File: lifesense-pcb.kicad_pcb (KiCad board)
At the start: 2 copper layers, 56 parts, among them CON1 USB-MINI-B, IC1 CC3000, J1 CONN_10X2, J4 CONN_10X2, P1 CONN_6, P2 CONN_01X01, P21 CONN_01X01, Q1 DTC114E, Q2 DTC114E, Q3 DTC114E, U1 TM4C123GH6PM, U2 TPS73633DRB, Y1 CRYSTAL, Y2 CRYSTAL

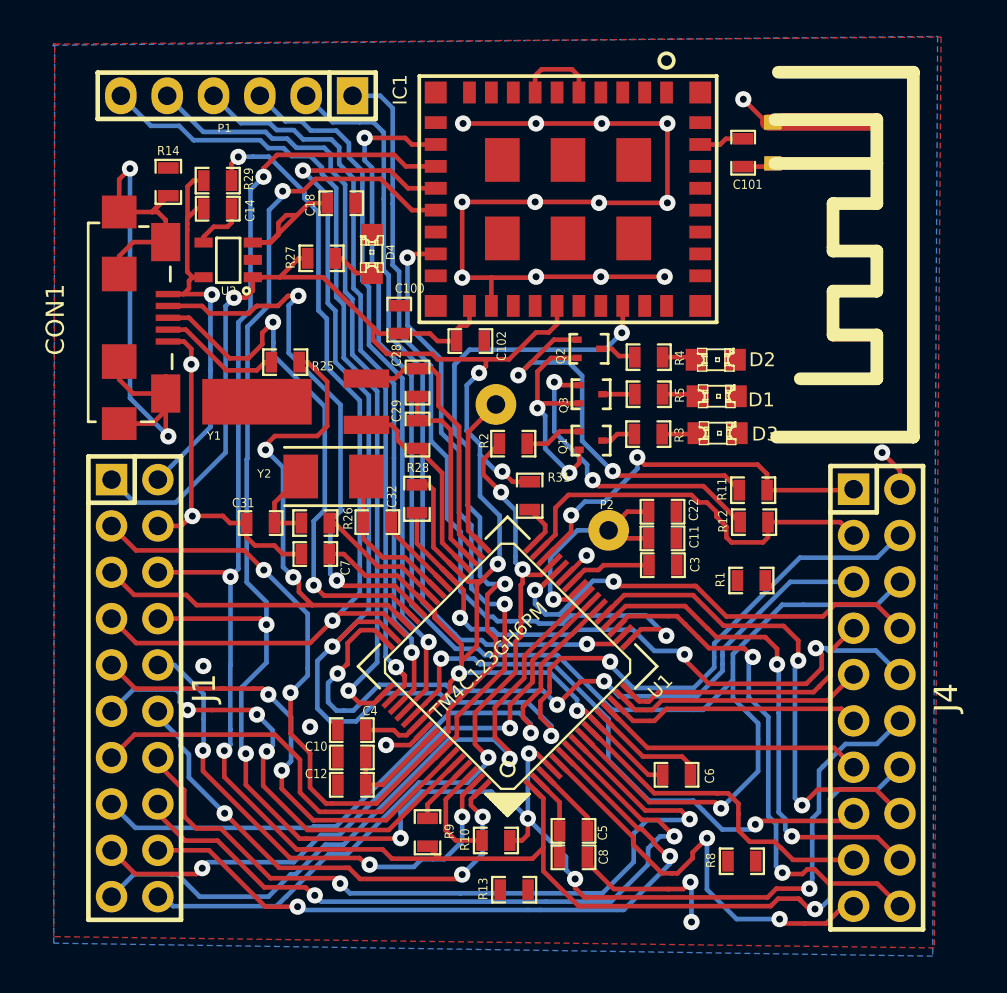
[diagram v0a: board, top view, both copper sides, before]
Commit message: finished board 1.0
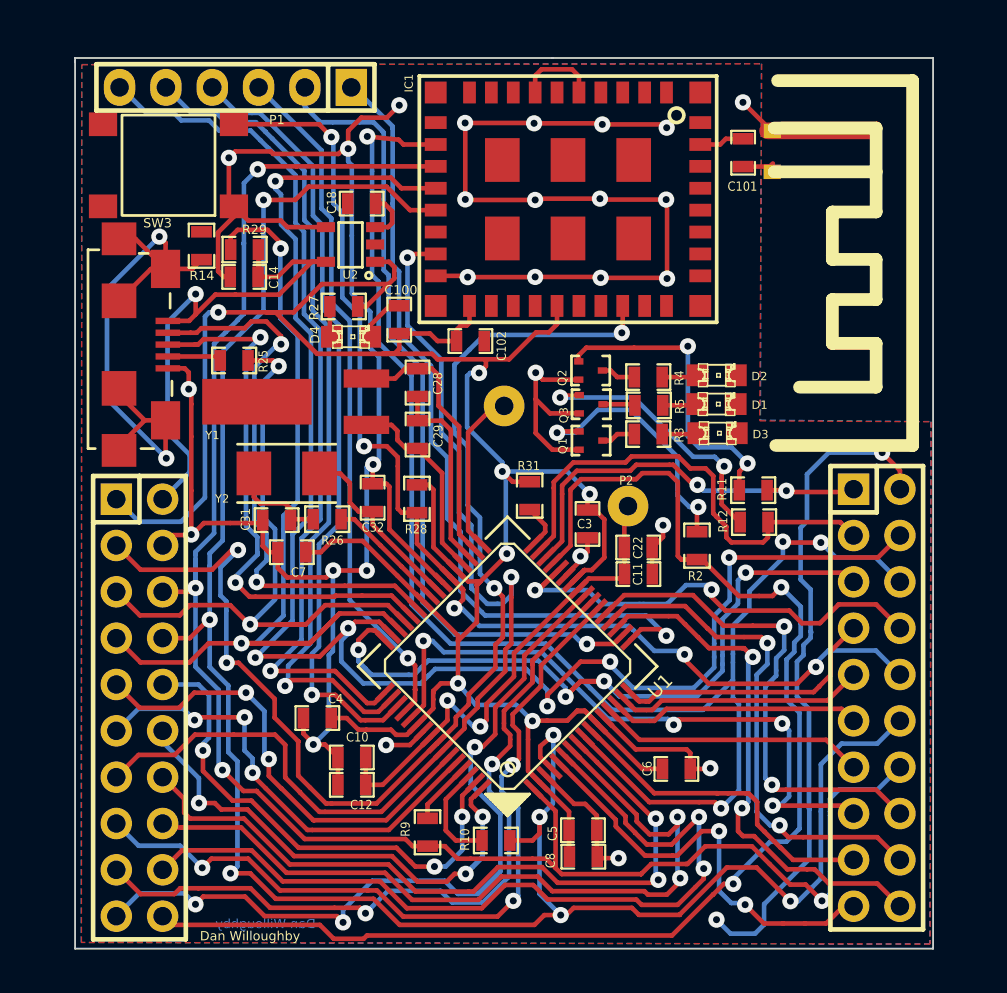
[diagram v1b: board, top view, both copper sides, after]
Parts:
- removed R1, R13: 0, lifesense:SMD-0603_r
- removed R8: 330, lifesense:SMD-0603_r
- added SW3: SW_PUSH, lifesense:B3S-1000, F.Cu at (133.9, 78.9)
- moved R2 11.5 mm to (162.9, 99.7), turned to 270 degrees
- moved U2 6.76 mm to (143.9, 83.2)
- moved C3 4.71 mm to (156.9, 98.5), turned to 270 degrees
- moved D4 4.68 mm to (144.0, 88.3), turned to 0 degrees
- moved R29 4.06 mm to (138.1, 83.5), turned to 180 degrees
- moved C14 4.01 mm to (138.1, 85.0), turned to 180 degrees
- moved R14 3.94 mm to (135.8, 83.3)
- moved R27 2.91 mm to (143.6, 86.6), turned to 180 degrees
- moved R25 2.80 mm to (137.6, 89.6)
- moved Y2 2.58 mm to (140.4, 95.8)
- moved C22 2.37 mm to (159.7, 99.8)
- moved C11 2.36 mm to (159.7, 101.3)
- moved C4 2.00 mm to (142.1, 109.2)
- moved P2 1.70 mm to (159.1, 97.6)
- moved CON1 1.47 mm to (131.2, 88.7)
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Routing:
- net GND: track 112.1 -> 217.2 mm, vias 22 -> 30
- net /LED_R: track 43.7 -> 74.1 mm, vias 3 -> 2
- net /~RST~: track 35.5 -> 65.1 mm, vias 3 -> 5
- net +3.3V: track 121.0 -> 144.9 mm, vias 6 -> 7
- net Net-(Q1-Pad1): track 3.13 -> 14.3 mm, vias 0 -> 2
- net /MOSI: track 112.5 -> 121.8 mm, vias 8 -> 7
- net /PA5: track 35.6 -> 43.7 mm, vias 1 -> 3
- net /PA6: track 34.5 -> 42.4 mm
- net /PE3: track 38.9 -> 46.7 mm
- net MCU_VDDC: track 19.7 -> 27.4 mm, vias 1 -> 2
- net USB_VBUS: track 22.8 -> 29.7 mm
- net Net-(CON1-Pad6): track 39.8 -> 33.1 mm
- net Net-(C18-Pad1): track 8.32 -> 2.75 mm
- net /PD6: track 32.1 -> 37.5 mm, vias 2 -> 4
- net /PA7: track 38.3 -> 43.4 mm, vias 1 -> 3
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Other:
- board outline added: 47 x 48.8 mm
- board text added: "Dan Willoughby"
